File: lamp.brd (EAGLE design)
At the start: 36.5 x 50.2 mm, 16 parts, among them IC1 LM358D, T2 TIP32C

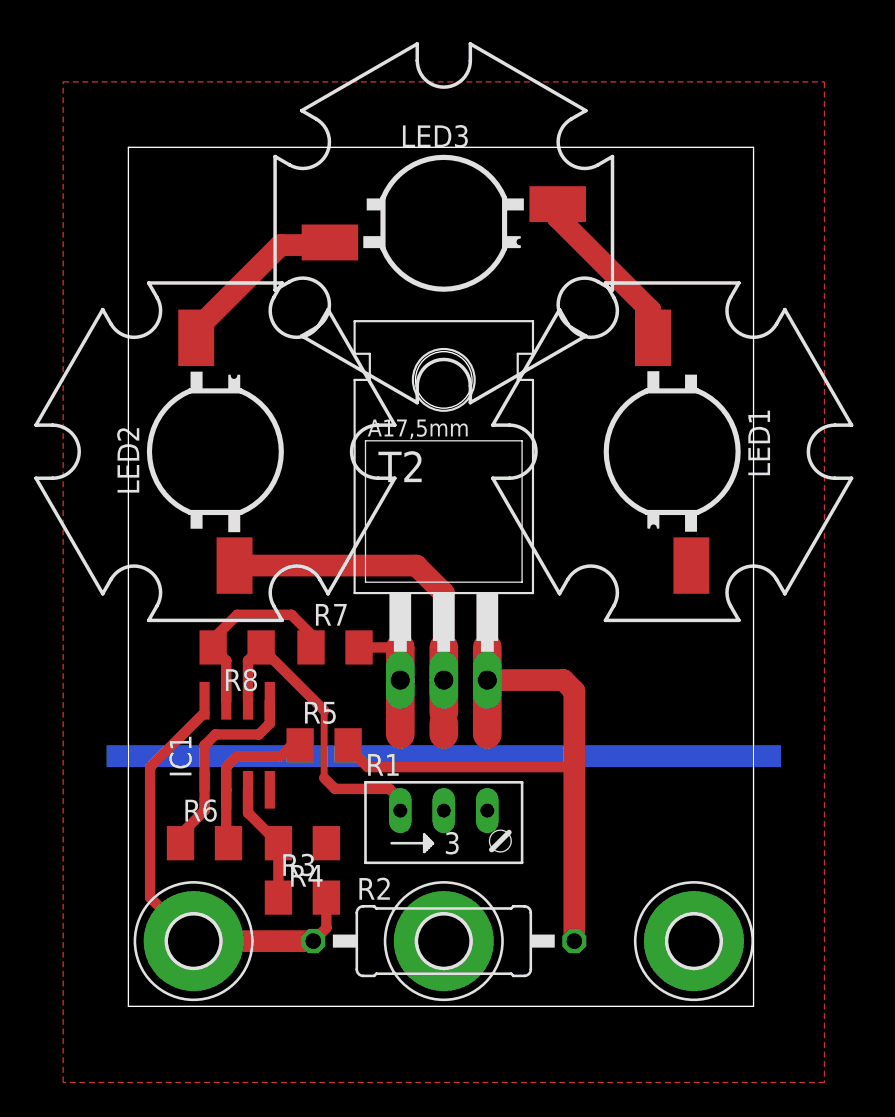
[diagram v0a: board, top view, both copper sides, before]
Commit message: Improved the design.
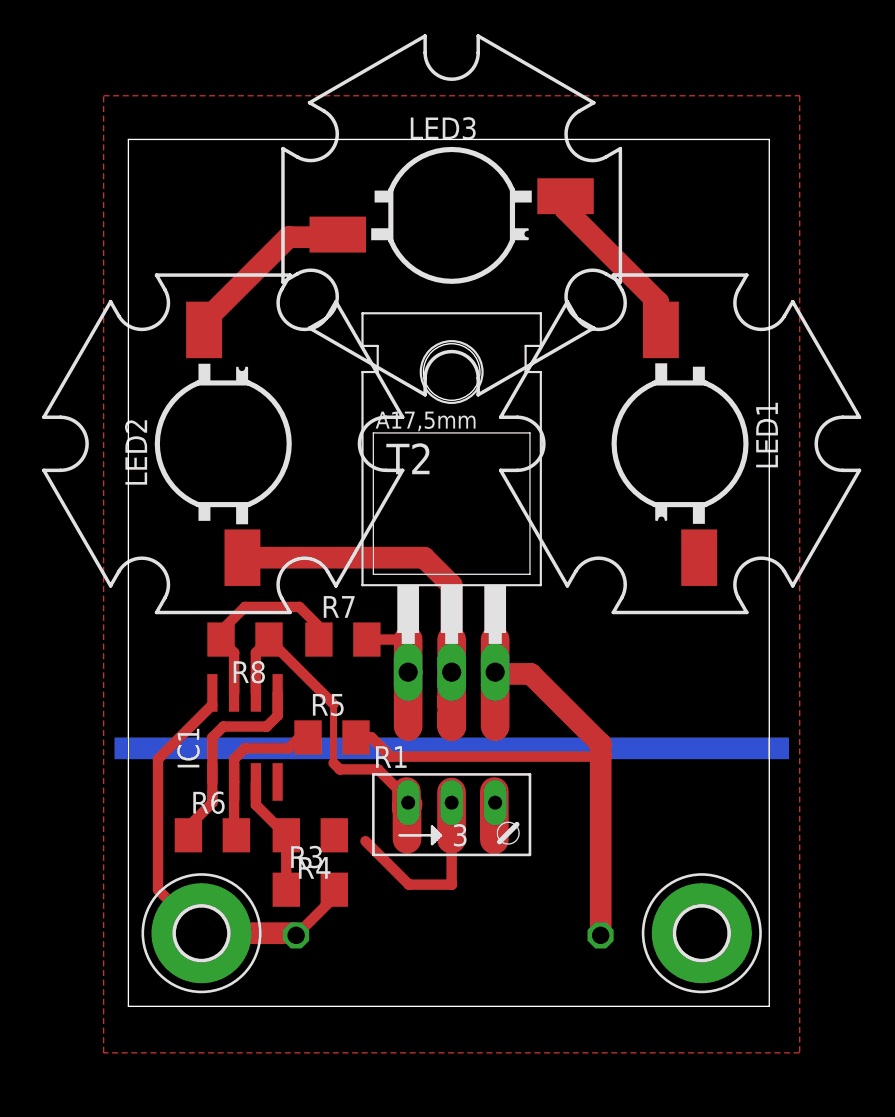
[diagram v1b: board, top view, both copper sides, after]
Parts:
- removed MOUNT: MOUNT-PAD-ROUND3.0, holes:3,0-PAD
- R2: device resistor:0411/15 -> resistor:0617/17
- moved T2 0.65 mm to (18.9, 25.9)
- moved R1 0.65 mm to (18.9, 11.3)
- moved R7 0.65 mm to (12.5, 21.4)
- moved R8 0.65 mm to (6.81, 21.4)
- moved LED3 0.65 mm to (18.9, 46.2)
- moved IC1 0.65 mm to (6.81, 15.7)
- moved R3 0.65 mm to (10.6, 6.81)
- moved R4 0.65 mm to (10.6, 9.99)
- moved R5 0.65 mm to (11.9, 15.7)
- moved R6 0.65 mm to (4.90, 9.99)
- moved VCC 0.65 mm to (4.27, 4.27)
- moved LED2 0.65 mm to (5.54, 32.8)
- moved GND 0.65 mm to (33.5, 4.27)
- moved LED1 0.65 mm to (32.2, 32.8)
- moved R2 0.43 mm to (18.7, 4.15), flipped to the bottom, turned to 180 degrees
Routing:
- net GND: track 0.00 -> 10.9 mm
- net N$20: track 0.00 -> 2.82 mm
- net N$19: track 0.00 -> 2.76 mm
- net N$13: track 0.00 -> 2.12 mm
- net N$15: track 0.00 -> 1.60 mm
- net N$18: track 0.00 -> 1.03 mm
- net VCC: track 26.2 -> 25.6 mm
- net N$10: track 18.2 -> 17.6 mm
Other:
- board size 36.5 x 50.2 mm -> 37.4 x 50.6 mm
